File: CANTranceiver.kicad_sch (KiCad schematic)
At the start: 8 parts, among them U3 IC TRANSCEIVER 1/1 8SO

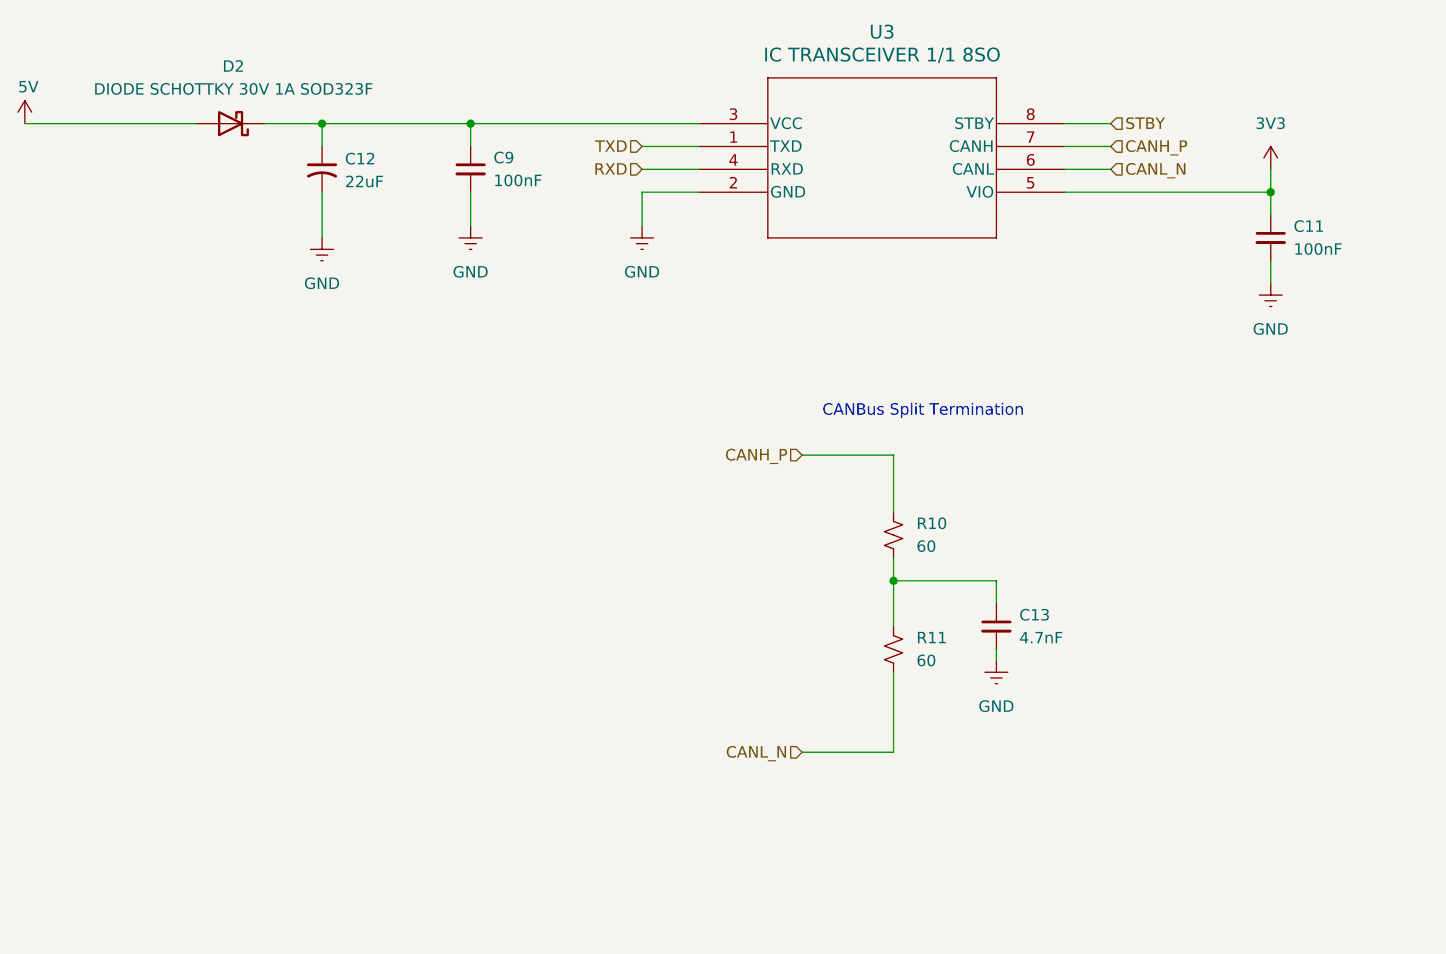
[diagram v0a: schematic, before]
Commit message: damir review
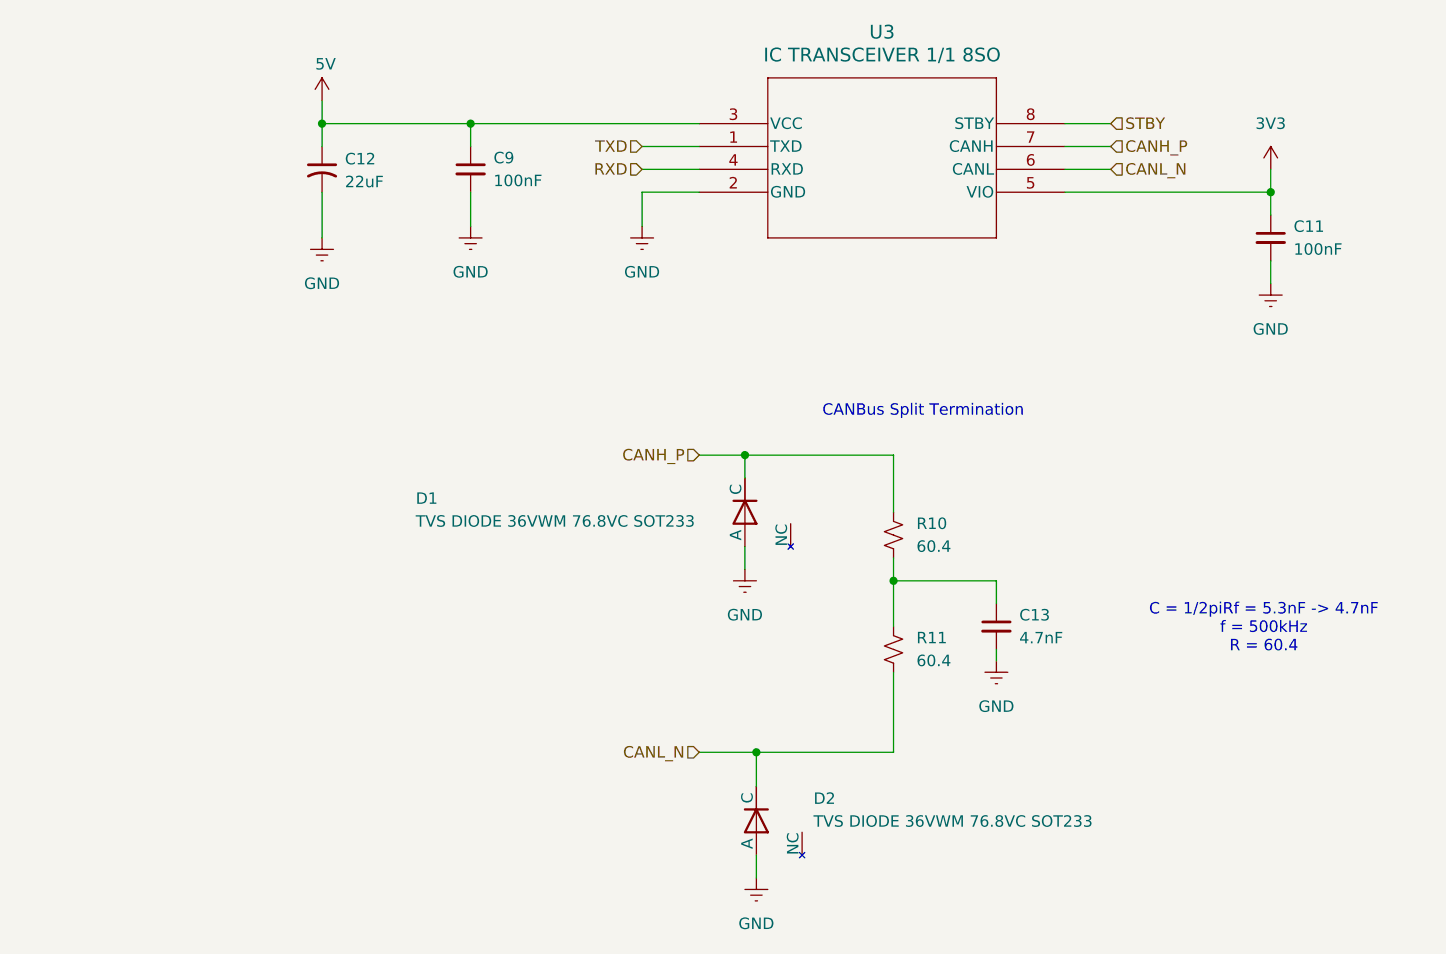
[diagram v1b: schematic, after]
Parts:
- removed D2: DIODE SCHOTTKY 30V 1A SOD323F, footprints:P39_SOD-323P, symbol symbols:SDB13HS-AQ
- added D1, D2: TVS DIODE 36VWM 76.8VC SOT233, footprints:P200_SOT-23, symbol symbols:Diode-NC_pin
- R10, R11: value 60 -> 60.4
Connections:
- net 5V: now also C12.1, C9.1, U3.3 (VCC)
- net CANH_P: now also D1.2 (C)
- net CANL_N: now also D2.2 (C)
- net GND: now also D1.1 (A), D2.1 (A)
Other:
- note added: "C = 1/2piRf = 5.3nF -> 4.7nF f = 500kHz R = 60.4"
